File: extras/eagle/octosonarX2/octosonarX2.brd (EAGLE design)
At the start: 68.6 x 45.7 mm, 47 parts, among them IC1 74HC125D, IC2 74HC125D, IC3 74HC125D, IC4 74HC125D, IC5 PCF8575C

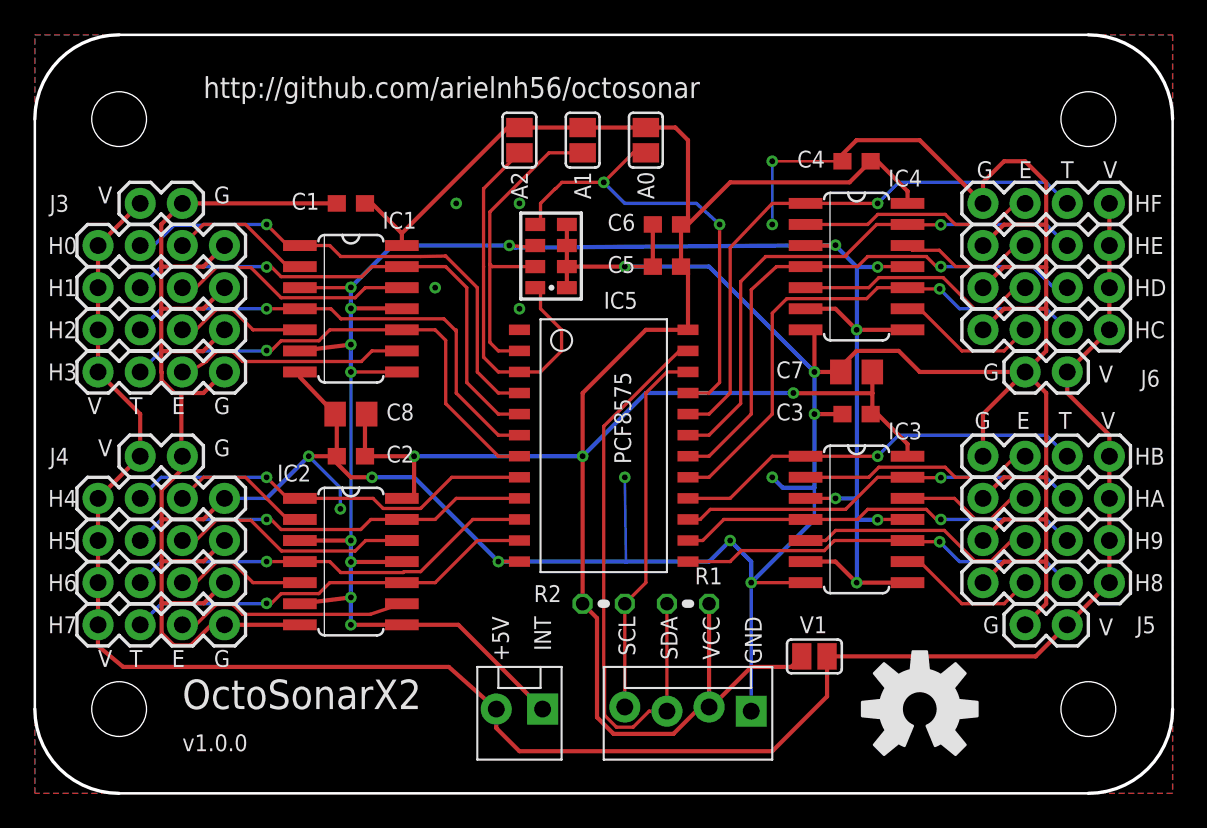
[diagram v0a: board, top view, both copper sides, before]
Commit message: Revert "Updates to X2 test and trimount bracket"
This reverts commit f0c77c11ce1398fcc169d7c2890869ee86536cf6.
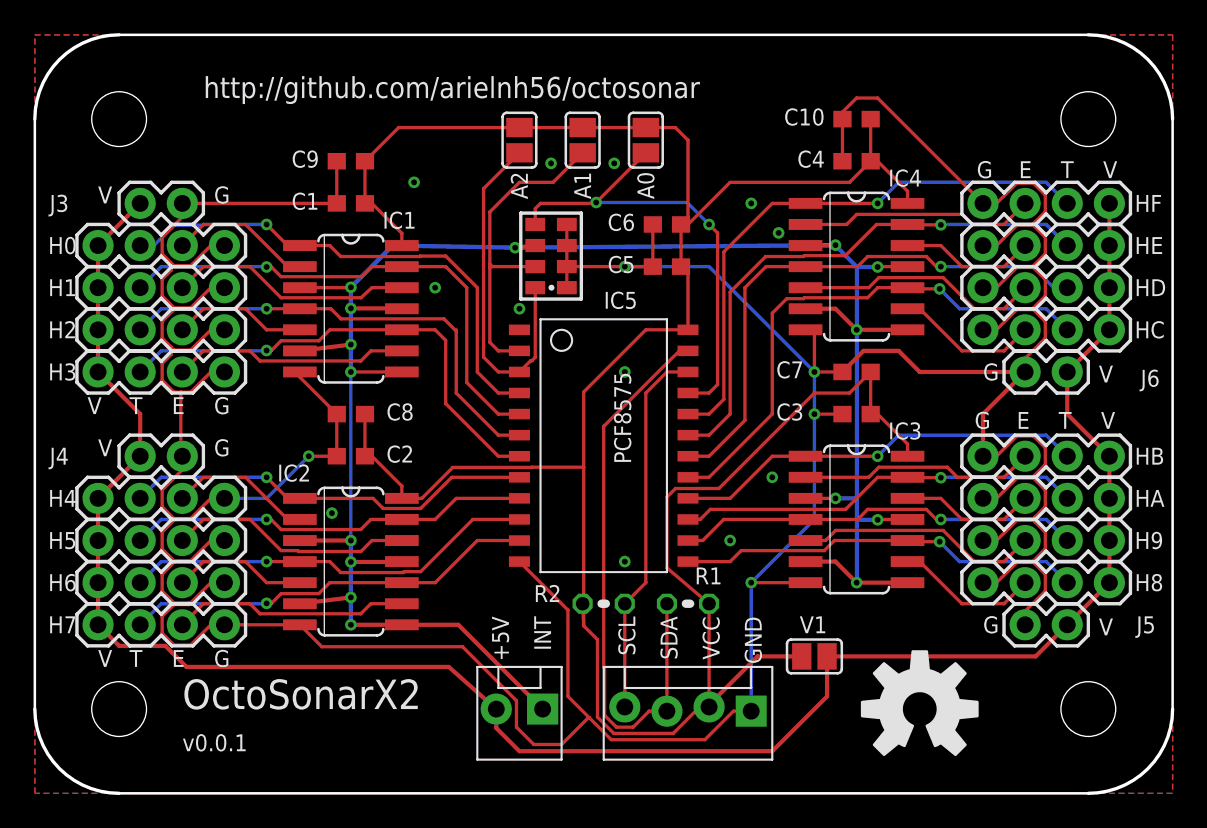
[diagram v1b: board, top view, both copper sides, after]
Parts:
- added C10, C9: 10uf, resistor:C0603
- C7, C8: device resistor:C0805 -> resistor:C0603
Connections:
- net GND: now also C10.2, C9.2
- net VCC: now also C10.1, C9.1
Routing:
- net VCC: track 146.1 -> 155.9 mm, vias 3 -> 0
- net GND: track 287.3 -> 282.2 mm
- net N$18: track 23.4 -> 21.3 mm
- net +5V: track 124.7 -> 123.8 mm
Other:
- board text added: "v0.0.1"
- board text removed: "v1.0.0"

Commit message: 1.2.0 eagle files and examples updated
Eagle files updated for OctoSonarX2 and Trimounts to reflect modifications between prototype and production.

OctoSonarX2 - tweaked bypass caps. Rerouted 5V with wider traces.
Examples - tidies up with serial only tests and separate LCD tests.
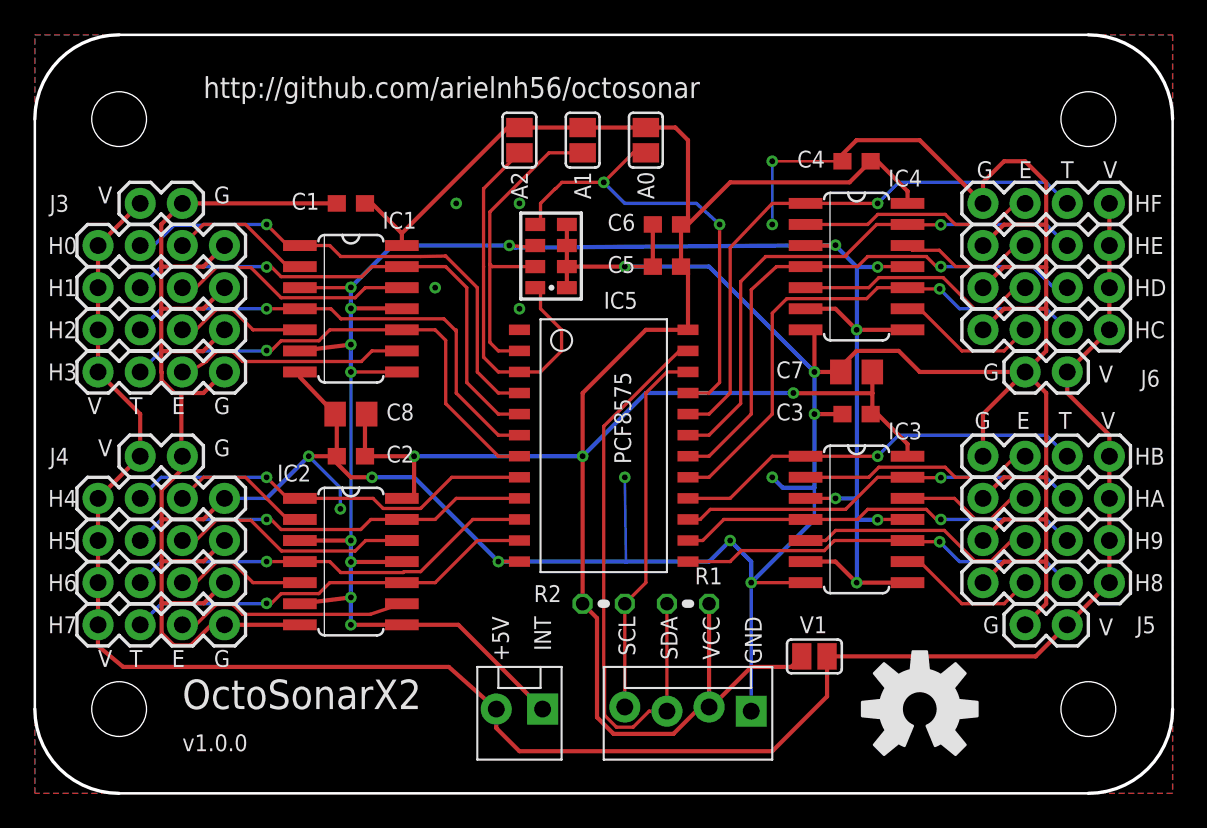
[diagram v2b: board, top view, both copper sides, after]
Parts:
- removed C10, C9: 10uf, resistor:C0603
- C7, C8: device resistor:C0603 -> resistor:C0805
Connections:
- net GND: no longer C10.2, C9.2
- net VCC: no longer C10.1, C9.1
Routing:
- net VCC: track 155.9 -> 146.1 mm, vias 0 -> 3
- net GND: track 282.2 -> 287.3 mm
- net N$18: track 21.3 -> 23.4 mm
- net +5V: track 123.8 -> 124.7 mm
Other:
- board text added: "v1.0.0"
- board text removed: "v0.0.1"
